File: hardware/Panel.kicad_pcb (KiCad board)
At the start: 2 copper layers, 65.3 x 64 mm, 33 parts, among them J101 Conn_01x02, J102 Header, J103 Header, J104 Conn_01x02, J201 Conn_01x02, J202 Conn_01x02, J203 SSD1306, SW101 Rotary Encoder + Switch, SW102 10mm, SW103 10mm, SW104 B3W-9000-RG2N, U101 XC6206P, U102 ATtiny4313

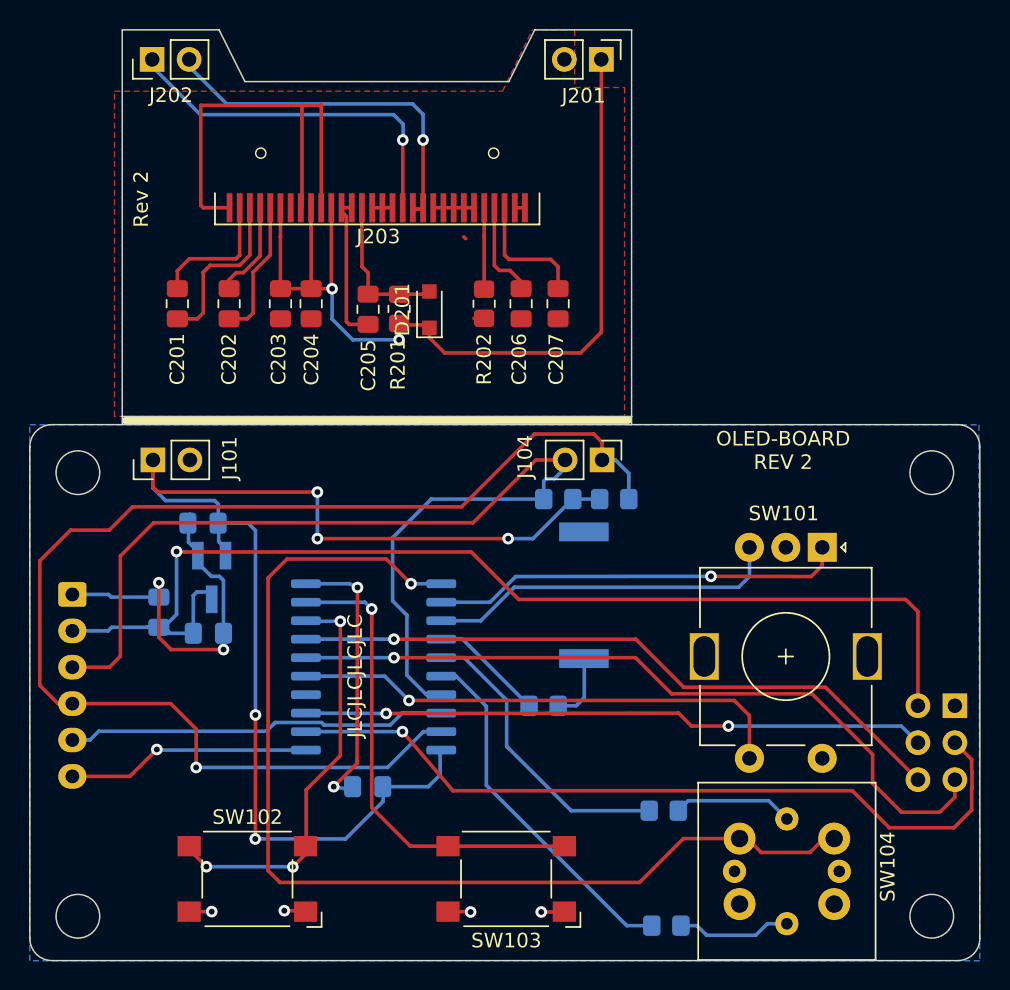
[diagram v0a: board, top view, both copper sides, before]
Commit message: KiCad 7.0 update
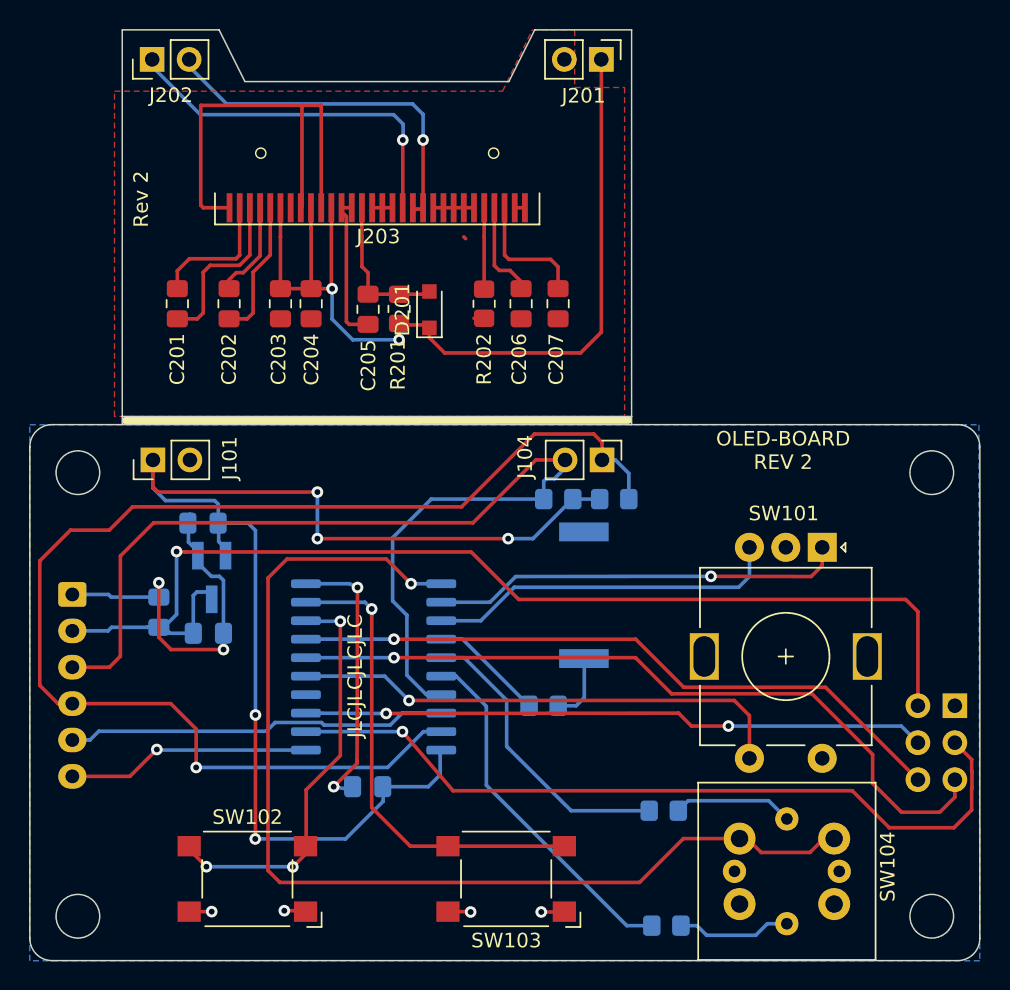
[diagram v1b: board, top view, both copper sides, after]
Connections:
- net ~INT renamed ~{INT}
- net ~RST renamed ~{RST}
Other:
- net class Default removed
- board text added: "~{INT}"
- board text added: "~{RST}"
- board text removed: "~INT"
- board text removed: "~RST"
